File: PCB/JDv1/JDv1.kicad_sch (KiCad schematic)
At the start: 0 parts

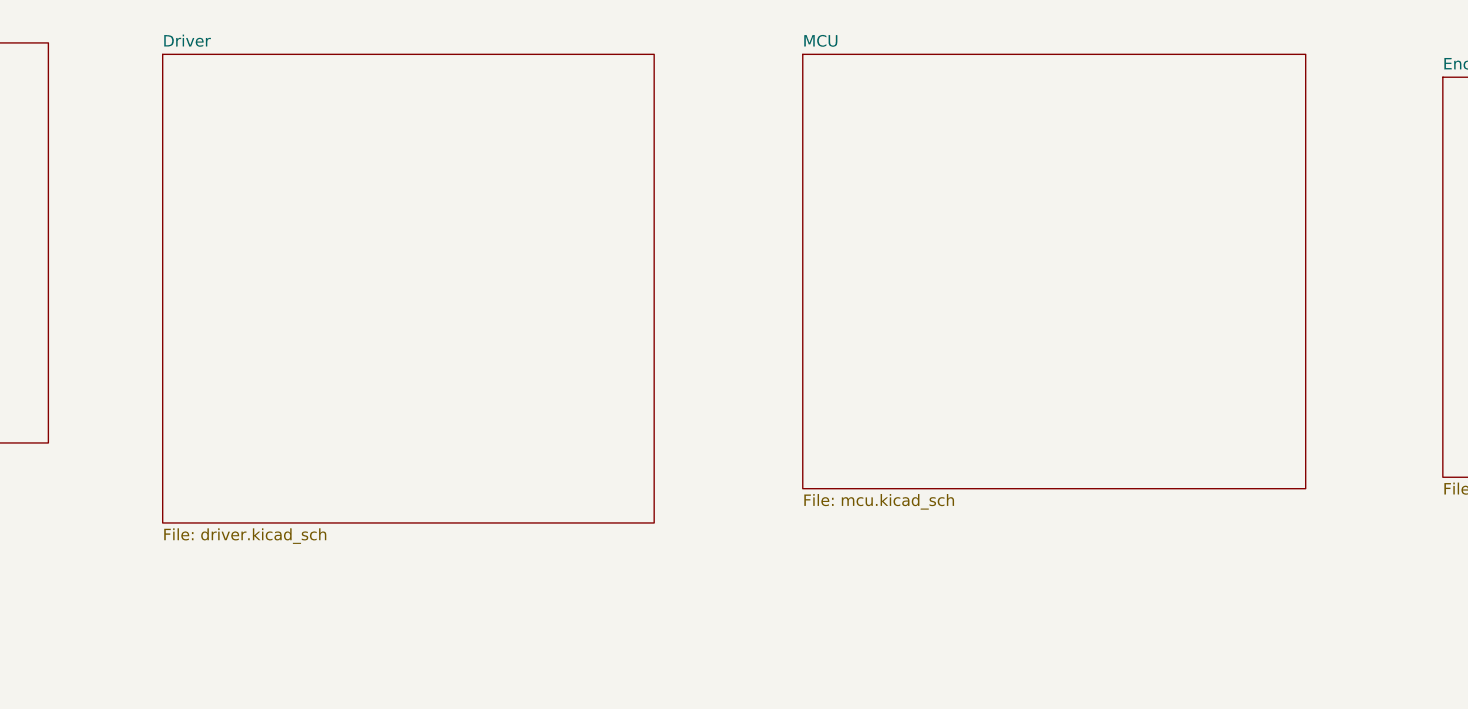
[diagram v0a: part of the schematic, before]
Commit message: syncing
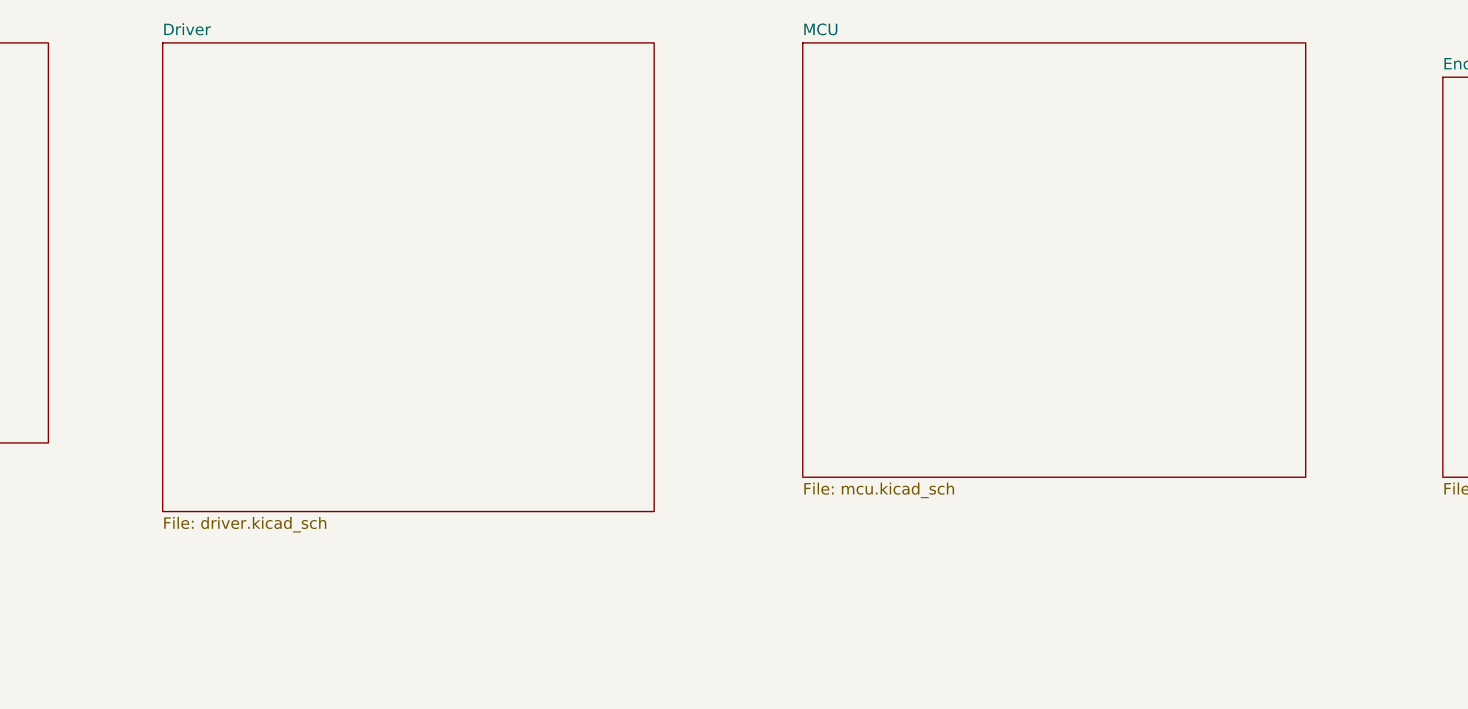
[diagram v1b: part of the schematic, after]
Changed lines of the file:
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@@
 	)
 	(sheet
-		(at 83.82 24.13)
+		(at 83.82 22.86)
 		(size 54.61 52.07)
 		(exclude_from_sim no)
@@
 		)
 		(property "Sheetname" "Driver"
-			(at 83.82 23.4184 0)
+			(at 83.82 22.1484 0)
 			(effects
 				(font
@@
 		)
 		(property "Sheetfile" "driver.kicad_sch"
-			(at 83.82 76.7846 0)
+			(at 83.82 75.5146 0)
 			(effects
 				(font
@@
 	)
 	(sheet
-		(at 154.94 24.13)
+		(at 154.94 22.86)
 		(size 55.88 48.26)
 		(exclude_from_sim no)
@@
 		)
 		(property "Sheetname" "MCU"
-			(at 154.94 23.4184 0)
+			(at 154.94 22.1484 0)
 			(effects
 				(font
@@
 		)
 		(property "Sheetfile" "mcu.kicad_sch"
-			(at 154.94 72.9746 0)
+			(at 154.94 71.7046 0)
 			(effects
 				(font
